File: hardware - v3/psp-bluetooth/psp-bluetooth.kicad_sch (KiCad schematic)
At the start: 22 parts, among them J1 Left Connector, J2 Center Connector, J3 Right Connector, J4 Analog Connector, J5 PSP Power out, J6 Barrel_Jack, J8 Vin Toggle, P1 Digital, P2 Analog, SW1 SW_Push, U1 MCP4251-xxxx-P

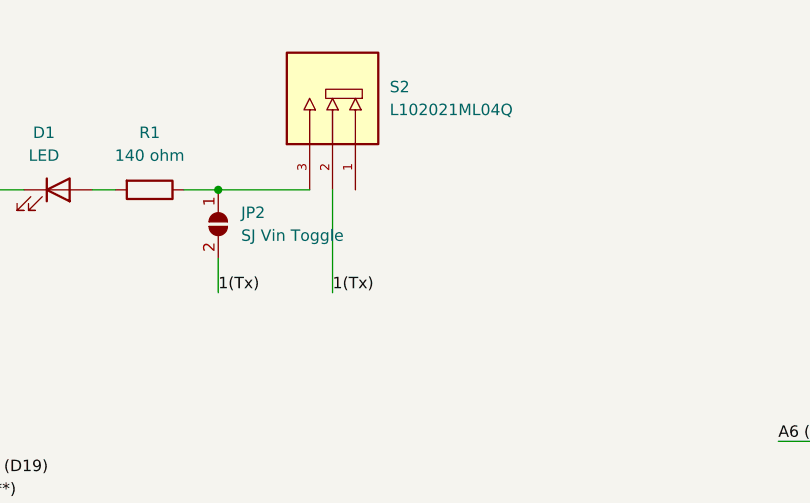
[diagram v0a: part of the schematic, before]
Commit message: Finished
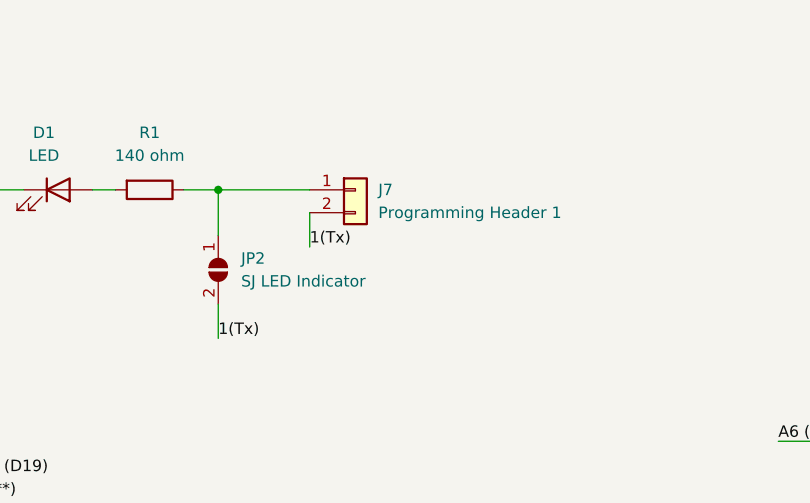
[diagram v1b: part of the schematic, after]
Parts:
- removed S2: L102021ML04Q, L102021ML04Q:SW_L102021ML04Q, symbol L102021ML04Q:L102021ML04Q
- added J7: Programming Header 1, Connector_PinHeader_2.54mm:PinHeader_1x02_P2.54mm_Vertical, symbol Connector_Generic:Conn_01x02
- JP2: value SJ Vin Toggle -> SJ LED Indicator
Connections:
- net 1(Tx): now also J7.2 (Pin_2)
- net at JP2.1 (A), R1.1: now also J7.1 (Pin_1)
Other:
- moved on the sheet: JP2
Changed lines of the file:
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@@
-    (stroke (width 0) (type default) (color 0 0 0 0))
-  )
-  (wire (pts (xy 121.92 31.75) (xy 121.92 43.18))
     (stroke (width 0) (type default) (color 0 0 0 0))
   )
@@
     (stroke (width 0) (type default) (color 0 0 0 0))
   )
-  (wire (pts (xy 109.22 39.37) (xy 109.22 43.18))
+  (wire (pts (xy 109.22 44.45) (xy 109.22 48.26))
     (stroke (width 0) (type default) (color 0 0 0 0))
   )
@@
   )
   (wire (pts (xy 43.18 69.85) (xy 41.91 69.85))
+    (stroke (width 0) (type default) (color 0 0 0 0))
+  )
+  (wire (pts (xy 119.38 38.1) (xy 119.38 34.29))
     (stroke (width 0) (type default) (color 0 0 0 0))
   )
@@
     (stroke (width 0) (type default) (color 0 0 0 0))
   )
+  (wire (pts (xy 109.22 36.83) (xy 109.22 31.75))
+    (stroke (width 0) (type default) (color 0 0 0 0))
+  )
   (wire (pts (xy 43.18 67.31) (xy 41.91 67.31))
     (stroke (width 0) (type default) (color 0 0 0 0))
@@
     (effects (font (size 1.524 1.524)) (justify left bottom))
   )
-  (label "1(Tx)" (at 109.22 43.18 0)
+  (label "1(Tx)" (at 109.22 48.26 0)
     (effects (font (size 1.27 1.27)) (justify left bottom))
   )
@@
     (effects (font (size 1.27 1.27)) (justify left bottom))
   )
-  (label "1(Tx)" (at 121.92 43.18 0)
+  (label "1(Tx)" (at 119.38 38.1 0)
     (effects (font (size 1.27 1.27)) (justify left bottom))
   )
@@
     (pin "2")
   )
-  (symbol (lib_id "L102021ML04Q:L102021ML04Q") (at 121.92 21.59 270) (mirror x) (unit 1)
-    (in_bom yes) (on_board yes) (fields_autoplaced)
-    (property "Reference" "S2" (id 0) (at 128.27 20.3199 90)
-      (effects (font (size 1.27 1.27)) (justify left))
-    )
-    (property "Value" "L102021ML04Q" (id 1) (at 128.27 22.8599 90)
-      (effects (font (size 1.27 1.27)) (justify left))
-    )
-    (property "Footprint" "L102021ML04Q:SW_L102021ML04Q" (id 2) (at 121.92 21.59 0)
-      (effects (font (size 1.27 1.27)) (justify left bottom) hide)
-    )
-    (property "Datasheet" "" (id 3) (at 121.92 21.59 0)
-      (effects (font (size 1.27 1.27)) (justify left bottom) hide)
-    )
-    (property "STANDARD" "Manufacturer Recommendations" (id 4) (at 121.92 21.59 0)
-      (effects (font (size 1.27 1.27)) (justify left bottom) hide)
-    )
-    (property "PARTREV" "N/A" (id 5) (at 121.92 21.59 0)
-      (effects (font (size 1.27 1.27)) (justify left bottom) hide)
-    )
-    (property "MAXIMUM_PACKAGE_HEIGHT" "7.92mm" (id 6) (at 121.92 21.59 0)
-      (effects (font (size 1.27 1.27)) (justify left bottom) hide)
-    )
-    (property "MANUFACTURER" "C&K" (id 7) (at 121.92 21.59 0)
-      (effects (font (size 1.27 1.27)) (justify left bottom) hide)
-    )
-    (pin "1")
-    (pin "2")
-    (pin "3")
-  )
   (symbol (lib_id "power:GND") (at 187.96 59.69 0) (unit 1)
     (in_bom yes) (on_board yes)
@@
     (pin "1")
   )
+  (symbol (lib_id "Connector_Generic:Conn_01x02") (at 124.46 31.75 0) (unit 1)
+    (in_bom yes) (on_board yes) (fields_autoplaced)
+    (property "Reference" "J7" (id 0) (at 127 31.7499 0)
+      (effects (font (size 1.27 1.27)) (justify left))
+    )
+    (property "Value" "Programming Header 1" (id 1) (at 127 34.2899 0)
+      (effects (font (size 1.27 1.27)) (justify left))
+    )
+    (property "Footprint" "Connector_PinHeader_2.54mm:PinHeader_1x02_P2.54mm_Vertical" (id 2) (at 124.46 31.75 0)
+      (effects (font (size 1.27 1.27)) hide)
+    )
+    (property "Datasheet" "~" (id 3) (at 124.46 31.75 0)
+      (effects (font (size 1.27 1.27)) hide)
+    )
+    (pin "1")
+    (pin "2")
+  )
   (symbol (lib_id "Connector_Generic:Conn_01x04") (at 173.99 173.99 0) (unit 1)
     (in_bom yes) (on_board yes) (fields_autoplaced)
@@
     (pin "1")
   )
-  (symbol (lib_id "Jumper:SolderJumper_2_Open") (at 109.22 35.56 90) (mirror x) (unit 1)
-    (in_bom yes) (on_board yes) (fields_autoplaced)
-    (property "Reference" "JP2" (id 0) (at 111.76 34.2899 90)
+  (symbol (lib_id "Jumper:SolderJumper_2_Open") (at 109.22 40.64 90) (mirror x) (unit 1)
+    (in_bom yes) (on_board yes) (fields_autoplaced)
+    (property "Reference" "JP2" (id 0) (at 111.76 39.3699 90)
       (effects (font (size 1.27 1.27)) (justify right))
     )
-    (property "Value" "SJ Vin Toggle" (id 1) (at 111.76 36.8299 90)
+    (property "Value" "SJ LED Indicator" (id 1) (at 111.76 41.9099 90)
       (effects (font (size 1.27 1.27)) (justify right))
     )
-    (property "Footprint" "Jumper:SolderJumper-2_P1.3mm_Open_Pad1.0x1.5mm" (id 2) (at 109.22 35.56 0)
-      (effects (font (size 1.27 1.27)) hide)
-    )
-    (property "Datasheet" "~" (id 3) (at 109.22 35.56 0)
+    (property "Footprint" "Jumper:SolderJumper-2_P1.3mm_Open_Pad1.0x1.5mm" (id 2) (at 109.22 40.64 0)
+      (effects (font (size 1.27 1.27)) hide)
+    )
+    (property "Datasheet" "~" (id 3) (at 109.22 40.64 0)
       (effects (font (size 1.27 1.27)) hide)
     )
@@
       (reference "J6") (unit 1) (value "Barrel_Jack") (footprint "Connector_BarrelJack:BarrelJack_CUI_PJ-063AH_Horizontal")
     )
+    (path "/ba7f31aa-9062-4aae-85d4-9505b7c62b96"
+      (reference "J7") (unit 1) (value "Programming Header 1") (footprint "Connector_PinHeader_2.54mm:PinHeader_1x02_P2.54mm_Vertical")
+    )
     (path "/c804af17-c55f-40bf-b2b9-46678ee29802"
       (reference "J8") (unit 1) (value "Vin Toggle") (footprint "Connector_PinHeader_2.54mm:PinHeader_1x02_P2.54mm_Vertical")
@@
     )
     (path "/c4009eaa-9387-4ecd-ba8f-391a4ed3d470"
-      (reference "JP2") (unit 1) (value "SJ Vin Toggle") (footprint "Jumper:SolderJumper-2_P1.3mm_Open_Pad1.0x1.5mm")
+      (reference "JP2") (unit 1) (value "SJ LED Indicator") (footprint "Jumper:SolderJumper-2_P1.3mm_Open_Pad1.0x1.5mm")
     )
     (path "/00000000-0000-0000-0000-000056d73fac"
@@
       (reference "S1") (unit 1) (value "L102021ML04Q") (footprint "L102021ML04Q:SW_L102021ML04Q")
     )
-    (path "/a9d5de95-f9fc-4bc9-8240-4dea9673b68c"
-      (reference "S2") (unit 1) (value "L102021ML04Q") (footprint "L102021ML04Q:SW_L102021ML04Q")
-    )
     (path "/a21946e4-4c39-4737-801b-2250133670ba"
